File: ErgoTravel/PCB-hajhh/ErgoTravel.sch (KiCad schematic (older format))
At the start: 70 parts, among them J1 , J10 AudioJack3_Ground, J11 AudioJack3_Ground, J2 , J3 , J4 , J5 , J6 , J7 , J8 , SW1 , SW10 , SW11 , SW12 , SW13 , SW14 , SW15 , SW16 , SW17 , SW18 , SW19 , SW2 , SW20 , SW21 , SW22 , SW23 , SW24 , SW25 , SW26 , SW27 , SW28 , SW29 RST, SW3 , SW30 , SW31 , SW4 , SW5 , SW6 , SW7 , SW8 , SW9 , U1 Promicro

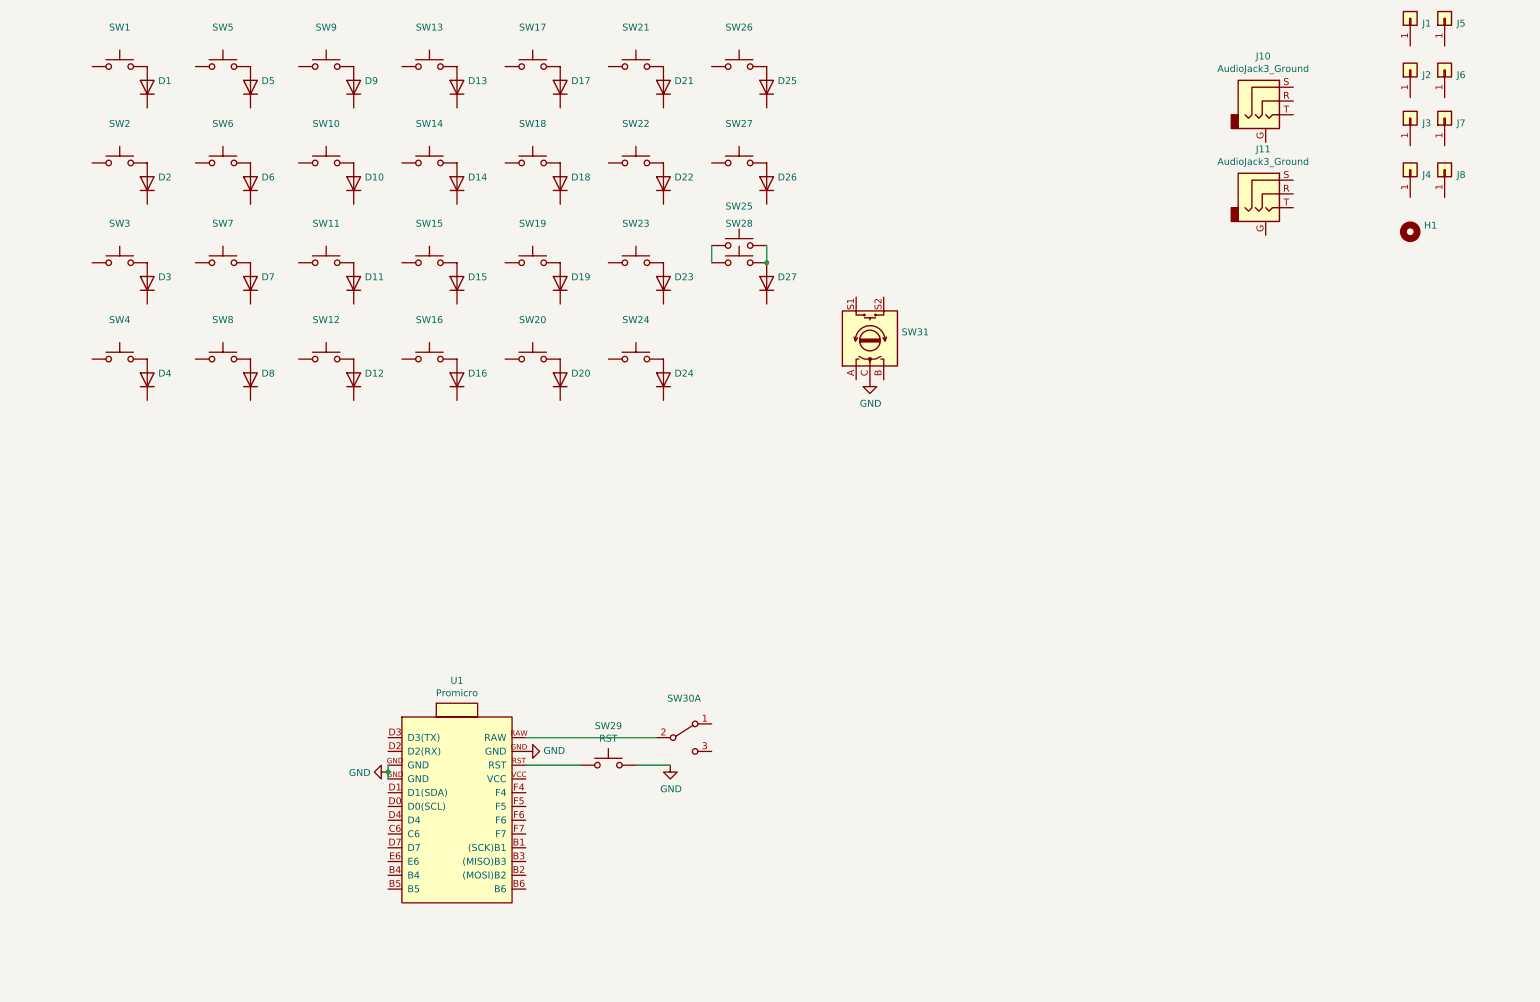
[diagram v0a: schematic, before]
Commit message: update 13:33 24/01/2021
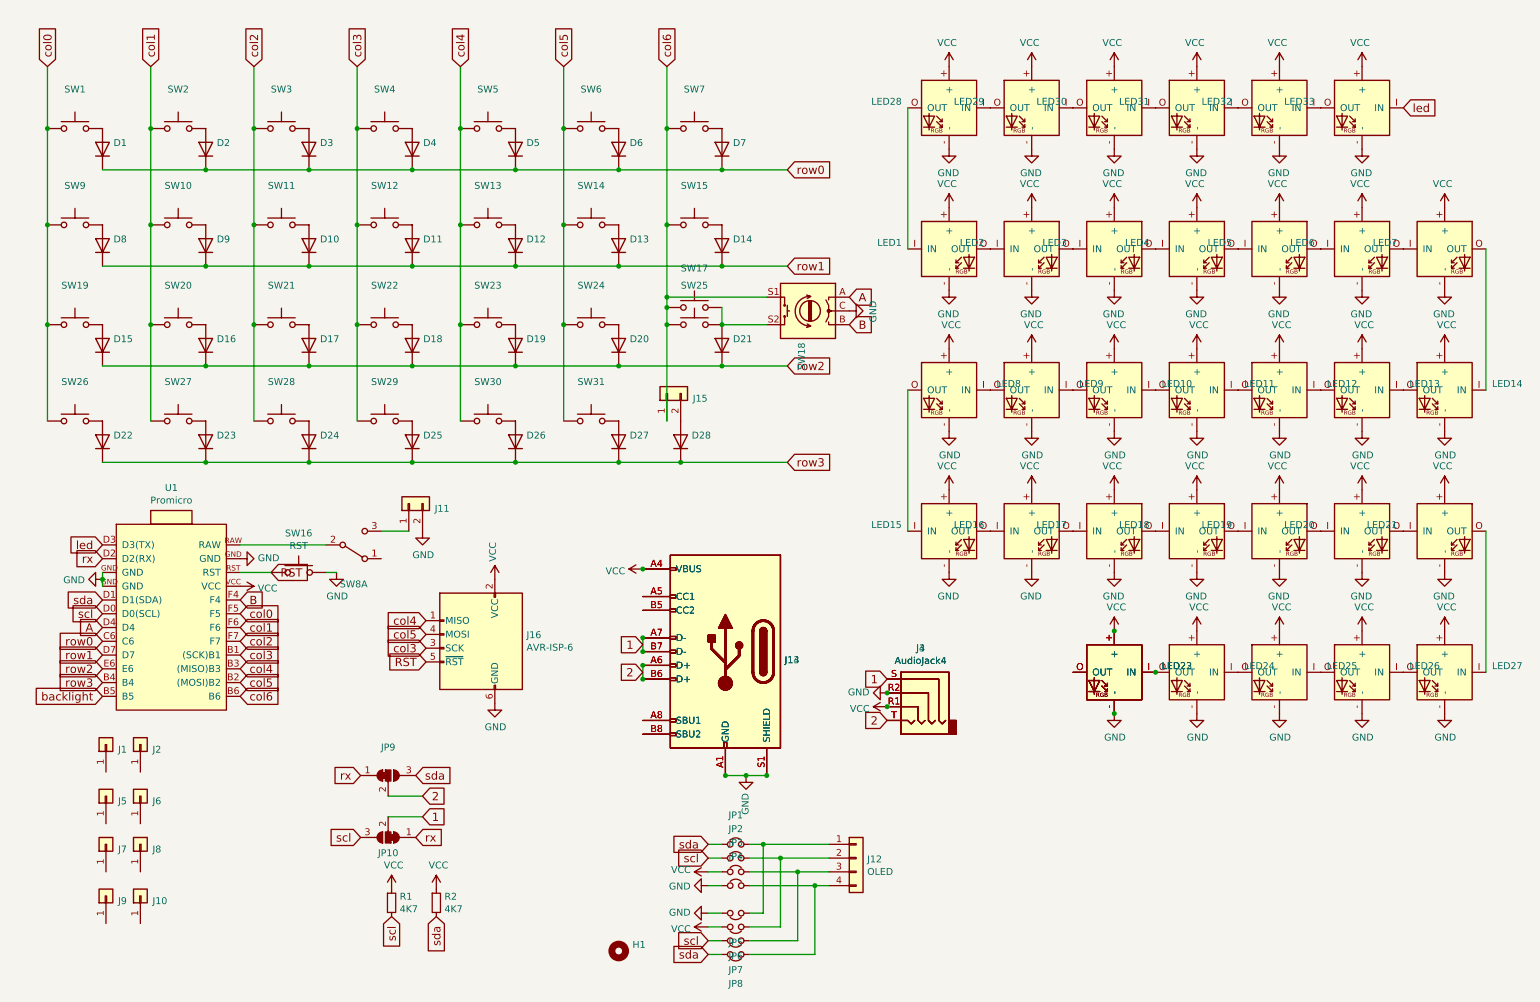
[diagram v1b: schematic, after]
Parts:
- removed J10, J11: AudioJack3_Ground, Connector_Audio:Jack_3.5mm_PJ320D_Horizontal, symbol Connector:AudioJack3_Ground
- added D28: (no value), fruitkt:DIODE, symbol Device:D
- added J11, J15: (no value), Connector_PinHeader_2.54mm:PinHeader_1x02_P2.54mm_Vertical, symbol Connector_Generic:Conn_01x02
- added J12: OLED, fruitkt:OLED-0.91, symbol Connector_Generic:Conn_01x04
- added J13, J14: (no value), fruitkt:USB-C-16pin-hight, symbol Connector:USB_C_Receptacle_USB2.0
- added J16: AVR-ISP-6, Connector_PinHeader_2.54mm:PinHeader_2x03_P2.54mm_Vertical, symbol Connector:AVR-ISP-6
- added J3, J4: AudioJack4, Connector_Audio:Jack_3.5mm_PJ320D_Horizontal, symbol Connector:AudioJack4
- added JP1, JP2, JP3, JP4, JP5, JP6, JP7, JP8: (no value), footprints:Jump, symbol Device:Jumper_NC_Small
- added JP10, JP9: (no value), Jumper:SolderJumper-3_P1.3mm_Bridged12_Pad1.0x1.5mm_NumberLabels, symbol Jumper:SolderJumper_3_Bridged12
- added LED1, LED15, LED16, LED17, LED18, LED19, LED2, LED20, LED23, LED3, LED4, LED5, LED6, LED7: (no value), footprints:SK6812mini-e-R2L, symbol fruitkt:6812
- added LED10, LED11, LED12, LED13, LED14, LED21, LED22, LED24, LED25, LED26, LED27, LED8, LED9: (no value), footprints:SK6812mini-e-L2R, symbol fruitkt:6812
- added LED28, LED29, LED30, LED31, LED32, LED33: (no value), fruitkt:SK6812MINI-FLIP, symbol fruitkt:6812
- added R1, R2: 4K7, Resistor_SMD:R_0805_2012Metric, symbol Device:R_Small
- D1, D10, D19: footprint (none) -> fruitkt:DIODE
- D11: renamed from D14; footprint (none) -> fruitkt:DIODE
- D12: renamed from D18; footprint (none) -> fruitkt:DIODE
- D13: renamed from D22; footprint (none) -> fruitkt:DIODE
- D14: renamed from D26; footprint (none) -> fruitkt:DIODE
- D15: renamed from D3; footprint (none) -> fruitkt:DIODE
- D16: renamed from D7; footprint (none) -> fruitkt:DIODE
- D17: renamed from D11; footprint (none) -> fruitkt:DIODE
- D18: renamed from D15; footprint (none) -> fruitkt:DIODE
- D2: renamed from D5; footprint (none) -> fruitkt:DIODE
- D20: renamed from D23; footprint (none) -> fruitkt:DIODE
- D21: renamed from D27; footprint (none) -> fruitkt:DIODE
- D22: renamed from D4; footprint (none) -> fruitkt:DIODE
- D23: renamed from D8; footprint (none) -> fruitkt:DIODE
- D24: renamed from D12; footprint (none) -> fruitkt:DIODE
- D25: renamed from D16; footprint (none) -> fruitkt:DIODE
- D26: renamed from D20; footprint (none) -> fruitkt:DIODE
- D27: renamed from D24; footprint (none) -> fruitkt:DIODE
- D3: renamed from D9; footprint (none) -> fruitkt:DIODE
- D4: renamed from D13; footprint (none) -> fruitkt:DIODE
- D5: renamed from D17; footprint (none) -> fruitkt:DIODE
- D6: renamed from D21; footprint (none) -> fruitkt:DIODE
- D7: renamed from D25; footprint (none) -> fruitkt:DIODE
- D8: renamed from D2; footprint (none) -> fruitkt:DIODE
- D9: renamed from D6; footprint (none) -> fruitkt:DIODE
- SW16: renamed from SW29; footprint Button_Switch_SMD:SW_SPST_TL3342 -> footprints:SW_TACT_ALPS_SKQGABE010
- SW8: renamed from SW30; footprint Button_Switch_SMD:SW_SPDT_PCM12 -> footprints:SW_SPDT_PCM12
- renumbered J8 to J10, J5 to J2, J2 to J5, J3 to J7, J7 to J8, J4 to J9, SW6 to SW10, SW10 to SW11, SW14 to SW12, SW18 to SW13, SW22 to SW14, SW27 to SW15, SW25 to SW17, SW31 to SW18, SW3 to SW19, SW5 to SW2, SW7 to SW20, SW11 to SW21, SW15 to SW22, SW19 to SW23, SW23 to SW24, SW28 to SW25, SW4 to SW26, SW8 to SW27, SW12 to SW28, SW16 to SW29, SW9 to SW3, SW20 to SW30, SW24 to SW31, SW13 to SW4, SW17 to SW5, SW21 to SW6, SW26 to SW7, SW2 to SW9
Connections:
- net GND: now also J11.2 (Pin_2), J13.A1 (GND), J13.A12 (GND), J13.B1 (GND), J13.B12 (GND), J13.S1 (SHIELD), J14.A1 (GND), J14.A12 (GND), J14.B1 (GND), J14.B12 (GND), J14.S1 (SHIELD), J16.6 (GND), J3.R2, J4.R2, JP4.1, JP5.1, LED1.-, LED10.-, LED11.-, LED12.-, LED13.-, LED14.-, LED15.-, LED16.-, LED17.-, LED18.-, LED19.-, LED2.-, LED20.-, LED21.-, LED22.-, LED23.-, LED24.-, LED25.-, LED26.-, LED27.-, LED28.-, LED29.-, LED3.-, LED30.-, LED31.-, LED32.-, LED33.-, LED4.-, LED5.-, LED6.-, LED7.-, LED8.-, LED9.-
- net col3: now reaches U1.B1 ((SCK)B1)
- net col3: now also SW12.1, SW22.1, SW29.1, SW4.1, J16.3 (SCK)
- net col5: now reaches U1.B2 ((MOSI)B2)
- net col5: now also SW14.1, SW24.1, SW31.1, SW6.1, J16.4 (MOSI)
- net col4: now reaches U1.B3 ((MISO)B3)
- net col4: now also SW13.1, SW23.1, SW30.1, SW5.1, J16.1 (MISO)
- net row3: now reaches U1.B4
- net row3: now also D22.1 (K), D23.1 (K), D24.1 (K), D25.1 (K), D26.1 (K), D27.1 (K), D28.1 (K)
- net backlight: now reaches U1.B5
- net col6: now reaches U1.B6
- net col6: now also SW15.1, SW17.1, SW18.S1, SW25.2, SW7.1, J15.1 (Pin_1)
- net row0: now reaches U1.C6
- net row0: now also D1.1 (K), D2.1 (K), D3.1 (K), D4.1 (K), D5.1 (K), D6.1 (K), D7.1 (K)
- net scl: now reaches U1.D0 (D0(SCL))
- net scl: now also JP10.3 (B), JP2.1, JP7.1, R1.2
- net sda: now reaches U1.D1 (D1(SDA))
- net sda: now also JP1.1, JP8.1, JP9.3 (B), R2.2
- net rx: now reaches U1.D2 (D2(RX))
- net rx: now also JP10.1 (A), JP9.1 (A)
- net led: now reaches U1.D3 (D3(TX))
- net led: now also LED33.I (IN)
- net A: now reaches U1.D4
- net A: now also SW18.A
- net row1: now reaches U1.D7
- net row1: now also D10.1 (K), D11.1 (K), D12.1 (K), D13.1 (K), D14.1 (K), D8.1 (K), D9.1 (K)
- net row2: now reaches U1.E6
- net row2: now also D15.1 (K), D16.1 (K), D17.1 (K), D18.1 (K), D19.1 (K), D20.1 (K), D21.1 (K)
- net B: now reaches U1.F4
- net B: now also SW18.B
- net col0: now reaches U1.F5
- net col0: now also SW1.1, SW19.1, SW26.1, SW9.1
- net col1: now reaches U1.F6
- net col1: now also SW10.1, SW2.1, SW20.1, SW27.1
- net col2: now reaches U1.F7
- net col2: now also SW11.1, SW21.1, SW28.1, SW3.1
- net RST: now reaches SW16.1, U1.RST
- net RST: now also J16.5 (~RST)
- net VCC: now reaches U1.VCC
- net VCC: now also J13.A4 (VBUS), J13.A9 (VBUS), J13.B4 (VBUS), J13.B9 (VBUS), J14.A4 (VBUS), J14.A9 (VBUS), J14.B4 (VBUS), J14.B9 (VBUS), J16.2 (VCC), J3.R1, J4.R1, JP3.1, JP6.1, LED1.+, LED10.+, LED11.+, LED12.+, LED13.+, LED14.+, LED15.+, LED16.+, LED17.+, LED18.+, LED19.+, LED2.+, LED20.+, LED21.+, LED22.+, LED23.+, LED24.+, LED25.+, LED26.+, LED27.+, LED28.+, LED29.+, LED3.+, LED30.+, LED31.+, LED32.+, LED33.+, LED4.+, LED5.+, LED6.+, LED7.+, LED8.+, LED9.+, R1.1, R2.1
- net at SW18.S2: now also D21.2 (A), SW17.2, SW25.1
- net at SW8.3 (C): now also J11.1 (Pin_1)
- new net: J12.1 (Pin_1), JP1.2, JP5.2
- new net: J12.2 (Pin_2), JP2.2, JP6.2
- new net: J12.3 (Pin_3), JP3.2, JP7.2
- new net: J12.4 (Pin_4), JP4.2, JP8.2
- new net: LED32.I (IN), LED33.O (OUT)
- new net: LED31.I (IN), LED32.O (OUT)
- new net: LED30.I (IN), LED31.O (OUT)
- new net: LED29.I (IN), LED30.O (OUT)
- new net: LED28.I (IN), LED29.O (OUT)
- new net: LED1.I (IN), LED28.O (OUT)
- new net: J13.A5 (CC1), J14.A5 (CC1)
- new net: J13.A8 (SBU1), J14.A8 (SBU1)
- new net: J13.B5 (CC2), J14.B5 (CC2)
- new net: J13.B8 (SBU2), J14.B8 (SBU2)
- new net: LED1.O (OUT), LED2.I (IN)
- new net: LED2.O (OUT), LED3.I (IN)
- new net: LED3.O (OUT), LED4.I (IN)
- new net: LED4.O (OUT), LED5.I (IN)
- new net: LED5.O (OUT), LED6.I (IN)
- new net: LED6.O (OUT), LED7.I (IN)
- new net: LED14.I (IN), LED7.O (OUT)
- new net: LED13.I (IN), LED14.O (OUT)
- new net: LED12.I (IN), LED13.O (OUT)
- new net: LED11.I (IN), LED12.O (OUT)
- new net: LED10.I (IN), LED11.O (OUT)
- new net: LED10.O (OUT), LED9.I (IN)
- new net: LED8.I (IN), LED9.O (OUT)
- new net: LED15.I (IN), LED8.O (OUT)
- new net: LED15.O (OUT), LED16.I (IN)
- new net: LED16.O (OUT), LED17.I (IN)
- new net: LED17.O (OUT), LED18.I (IN)
- new net: LED18.O (OUT), LED19.I (IN)
- new net: LED19.O (OUT), LED20.I (IN)
- new net: LED20.O (OUT), LED21.I (IN)
- new net: LED21.O (OUT), LED27.I (IN)
- new net: LED26.I (IN), LED27.O (OUT)
- new net: LED25.I (IN), LED26.O (OUT)
- new net: LED24.I (IN), LED25.O (OUT)
- new net: LED22.I (IN), LED23.I (IN), LED24.O (OUT)
- new net: LED22.O (OUT), LED23.O (OUT)
- new net: D28.2 (A), J15.2 (Pin_2)
- new net 1: J13.A7 (D-), J13.B7 (D-), J14.A7 (D-), J14.B7 (D-), J3.S, J4.S, JP10.2 (C)
- new net 2: J13.A6 (D+), J13.B6 (D+), J14.A6 (D+), J14.B6 (D+), J3.T, J4.T, JP9.2 (C)
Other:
- moved on the sheet: D1, D10, D11, D12, D13, D14, D15, D16, D17, D18, D19, D2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
